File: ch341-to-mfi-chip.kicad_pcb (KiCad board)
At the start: 2 copper layers, 23.5 x 18.4 mm, 14 parts, among them J1 USB-212-BCW, U1 CH341F, U2 HR1117V-3.3, U3 MFI337S3959

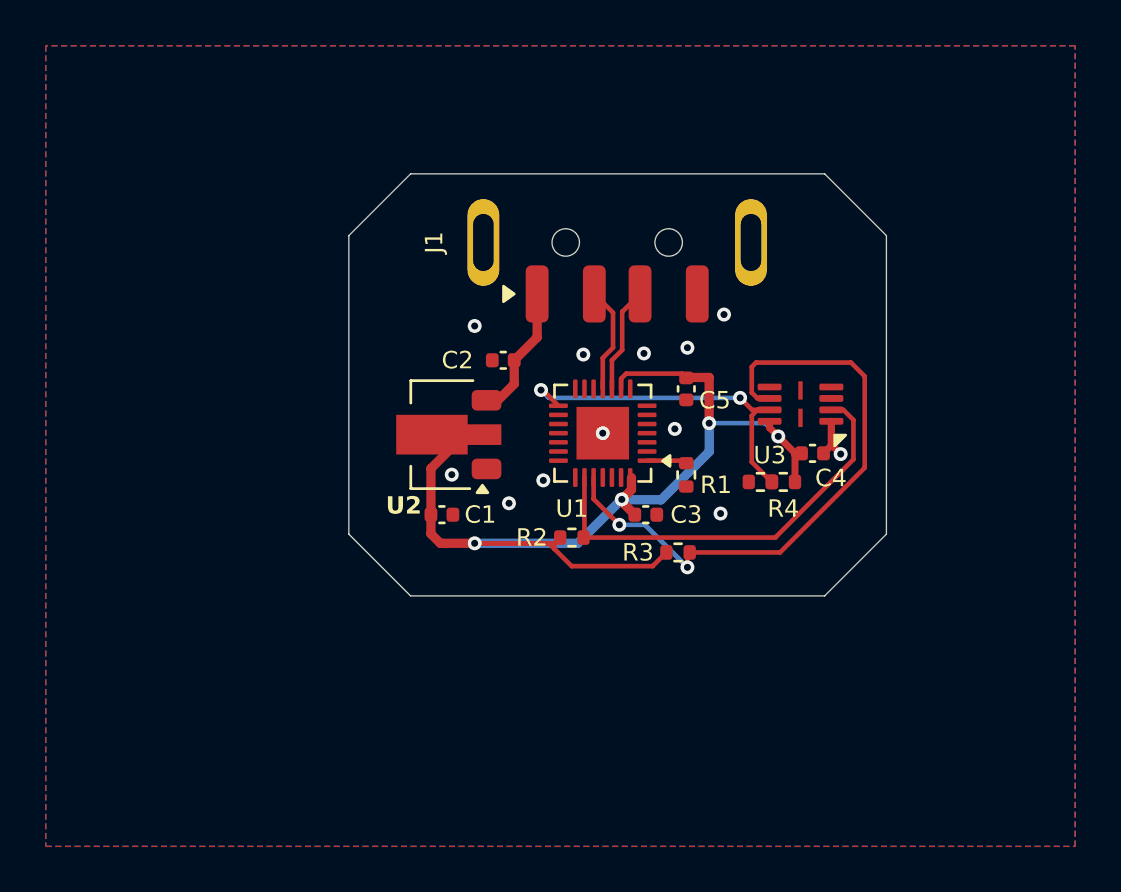
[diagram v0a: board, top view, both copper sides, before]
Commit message: now better
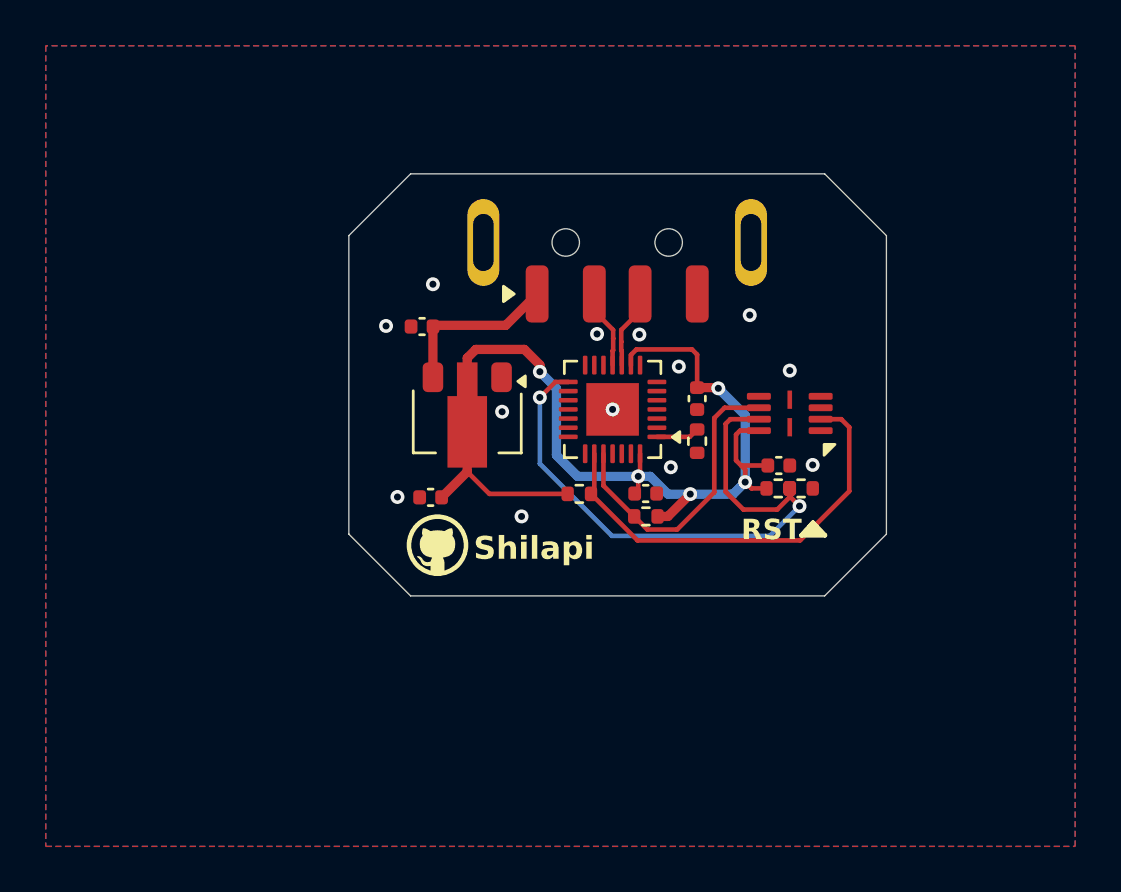
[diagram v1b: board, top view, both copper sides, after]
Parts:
- added G***: LOGO, KicadLibrary:GITHUB LOGO, F.Cu at (67.1, 54.4)
- moved C2 3.84 mm to (66.5, 44.8)
- moved R3 2.11 mm to (76.2, 53.1), turned to 180 degrees
- moved R2 1.94 mm to (73.3, 52.1)
- moved R5 1.80 mm to (83.0, 51.9), turned to 0 degrees
- moved C4 1.57 mm to (82.0, 50.9)
- moved R1 1.55 mm to (78.5, 49.8)
- moved U2 1.24 mm to (68.4, 48.9), turned to -90 degrees
- moved U1 1.13 mm to (74.8, 48.4)
- moved C3 0.93 mm to (76.2, 52.1)
- moved C1 0.91 mm to (66.8, 52.2), turned to 180 degrees
- moved C5 0.64 mm to (78.5, 47.9)
- moved U3 0.62 mm to (82.5, 48.6)
- moved R4 0.36 mm to (82.0, 51.9), turned to 0 degrees
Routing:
- net Net-(U1-SCL): track 27.4 -> 13.1 mm, vias 2 -> 0
- net Net-(U1-CS0): track 15.5 -> 26.8 mm
- net GND: track 3.14 -> 0.00 mm, vias 12 -> 13
- net Net-(J1-VBUS): track 5.36 -> 7.39 mm
- net +3V3: track 49.9 -> 48.2 mm, vias 4 -> 5
- net /USB_D-: track 4.68 -> 3.46 mm
- net /USB_D+: track 4.66 -> 3.46 mm
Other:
- board text added: "RST"
- board text added: "Shilapi"
